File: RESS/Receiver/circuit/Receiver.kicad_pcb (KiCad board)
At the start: 2 copper layers, 95.3 x 72.4 mm, 18 parts, among them J3 ADP_L, J4 ADP_R, J5 Power, J6 RESS_OUT1, SW2 SW_DIP_x02, U1 TLP785, U2 RR-1A, U3 48033S, U4 TC74HC32AP, U5 TC74HC08AP

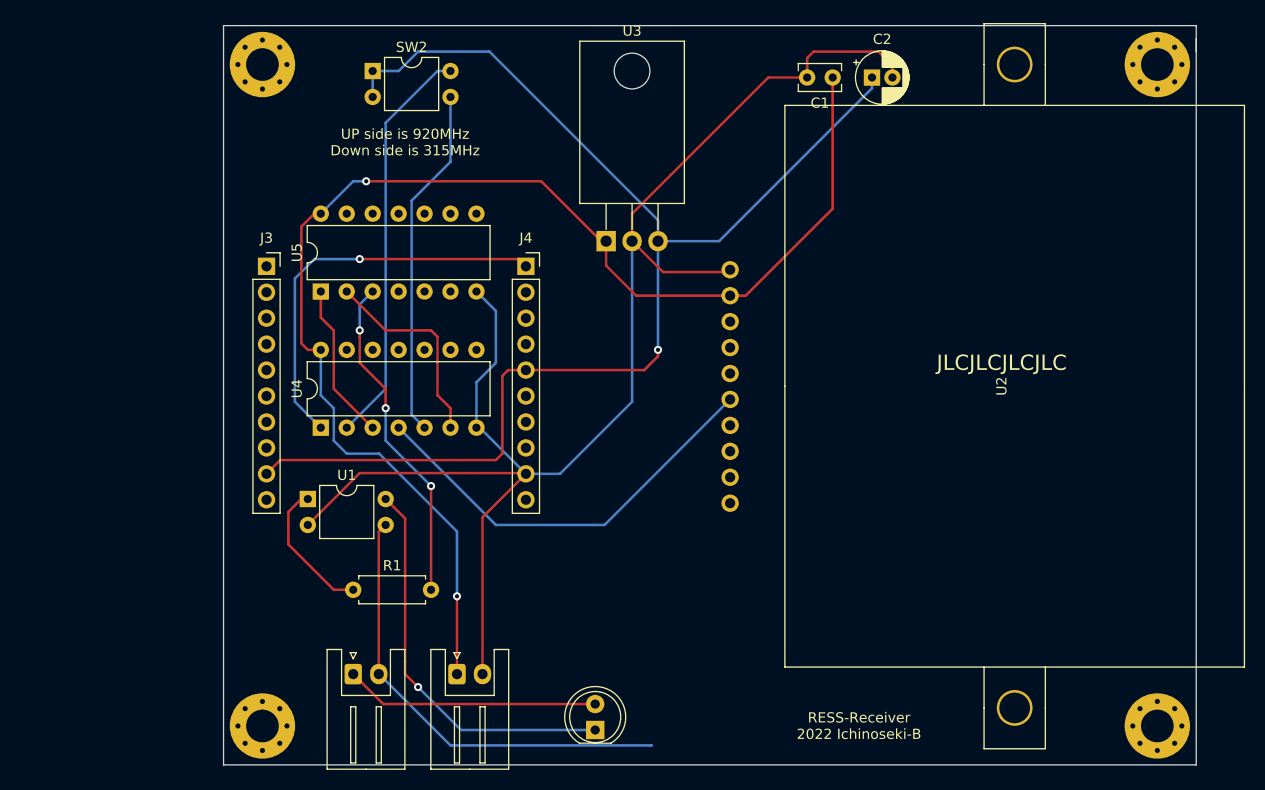
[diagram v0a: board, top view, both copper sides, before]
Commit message: WIP
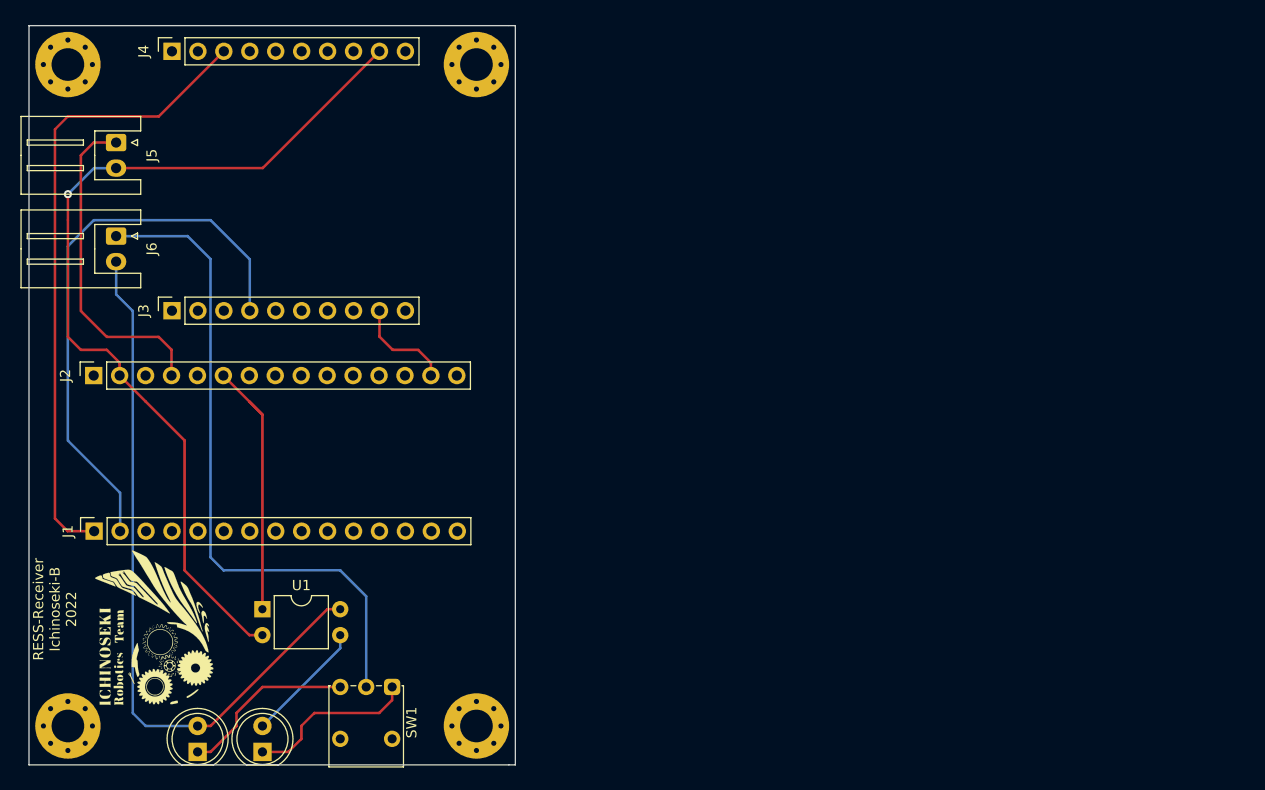
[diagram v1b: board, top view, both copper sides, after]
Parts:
- removed C1: 0.33μF, Capacitor_THT:C_Rect_L4.0mm_W2.5mm_P2.50mm
- removed C2: 47μF, Capacitor_THT:CP_Radial_D5.0mm_P2.00mm
- removed R1: 220Ω, Resistor_THT:R_Axial_DIN0207_L6.3mm_D2.5mm_P7.62mm_Horizontal
- removed SW2: SW_DIP_x02, Package_DIP:DIP-4_W7.62mm
- removed U2: RR-1A, RR1A:RR-1A
- removed U3: 48033S, Package_TO_SOT_THT:TO-220-3_Horizontal_TabDown
- removed U4: TC74HC32AP, Package_DIP:DIP-14_W7.62mm
- removed U5: TC74HC08AP, Package_DIP:DIP-14_W7.62mm
- added D2: LED, LED_THT:LED_D5.0mm, F.Cu at (97.8, 151.1)
- added J1: Conn_01x15_Female, Connector_PinSocket_2.54mm:PinSocket_1x15_P2.54mm_Vertical, F.Cu at (87.7, 129.5)
- added J2: Conn_01x15_Female, Connector_PinSocket_2.54mm:PinSocket_1x15_P2.54mm_Vertical, F.Cu at (87.6, 114.3)
- added J8: Logo, INCT:INCT, F.Cu at (92.7, 139.7)
- added SW1: SW_SPDT, Button_Switch_THT:SW_Push_1P2T_Vertical_E-Switch_800UDP8P1A1M6, F.Cu at (116.8, 144.8)
- J5: value Power -> Power_IN
- moved H3 66.7 mm to (125.1, 148.6)
- moved H4 66.7 mm to (125.1, 83.8)
- moved J5 61.8 mm to (89.8, 91.5), turned to -90 degrees
- moved J6 48.8 mm to (89.8, 100.6), turned to -90 degrees
- moved J4 40.6 mm to (95.3, 82.5), turned to 90 degrees
- moved D1 32.7 mm to (104.1, 151.1)
- moved H1 19.0 mm to (85.1, 83.8)
- moved H2 19.0 mm to (85.1, 148.6)
- moved U1 11.7 mm to (104.1, 137.2)
- moved J3 10.2 mm to (95.3, 107.9), turned to 90 degrees
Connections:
- J3 pad 1: (no net) -> Net-(J3-Pad1)
- J3 pad 10: (no net) -> Net-(J3-Pad10)
- J3 pad 2: (no net) -> Net-(J3-Pad2)
- J3 pad 3: (no net) -> Net-(J3-Pad3)
- J3 pad 4: (no net) -> RX
- J3 pad 5: (no net) -> Net-(J3-Pad5)
- J3 pad 6: (no net) -> Net-(J3-Pad6)
- J3 pad 7: (no net) -> Net-(J3-Pad7)
- J3 pad 8: (no net) -> Net-(J3-Pad8)
- J4 pad 1: OUT1 -> Net-(J4-Pad1)
- J4 pad 10: (no net) -> Net-(J4-Pad10)
- J4 pad 2: (no net) -> Net-(J4-Pad2)
- J4 pad 3: (no net) -> TX
- J4 pad 4: (no net) -> Net-(J4-Pad4)
- J4 pad 5: +3V3 -> Net-(J4-Pad5)
- J4 pad 6: (no net) -> Net-(J4-Pad6)
- J4 pad 7: (no net) -> Net-(J4-Pad7)
- J4 pad 8: (no net) -> Net-(J4-Pad8)
- J6 pad 1: Net-(D1-Pad2) -> Net-(J6-Pad1)
- J6 pad 2: Net-(J6-Pad2) -> Net-(D2-Pad2)
- U1 pad 1: Net-(R1-Pad1) -> Out
- U1 pad 3: Net-(J6-Pad2) -> Net-(D1-Pad2)
- U1 pad 4: Net-(D1-Pad1) -> Net-(D2-Pad2)
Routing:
- net +3V3: track 127.2 -> 9.90 mm, vias 1 -> 0
- net +5V: track 129.0 -> 32.2 mm, vias 2 -> 0
- net Net-(D2-Pad2): track 0.00 -> 70.5 mm
- net Net-(J6-Pad1): track 0.00 -> 65.1 mm
- net TX: track 0.00 -> 62.2 mm
- net RX: track 0.00 -> 55.5 mm
- net GND: track 144.0 -> 89.6 mm, vias 0 -> 1
- net Net-(J6-Pad2): track 44.5 -> 0.00 mm
- net OUT2: track 41.5 -> 0.00 mm
- net OUT1: track 40.0 -> 0.00 mm, vias 1 -> 0
- net OUT3: track 39.9 -> 0.00 mm
- net OUT4: track 34.5 -> 0.00 mm
- net OUT: track 32.6 -> 0.00 mm, vias 3 -> 0
- net Out: track 0.00 -> 26.3 mm
- net Net-(D1-Pad1): track 38.8 -> 16.8 mm, vias 1 -> 0
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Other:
- board size 95.3 x 72.4 mm -> 47.6 x 72.4 mm
- net class Default removed
- board text added: "JLCJLCJLC"
- board text added: "RESS-Receiver Ichinoseki-B 2022"
- board text removed: "JLCJLCJLCJLC"
- board text removed: "RESS-Receiver 2022 Ichinoseki-B"
- board text removed: "UP side is 920MHz Down side is 315MHz"
